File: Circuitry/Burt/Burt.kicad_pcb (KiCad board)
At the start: 2 copper layers, 111.1 x 114.2 mm, 41 parts, among them J1 Conn_01x20, J2 Conn_01x08_Female, M1 Motor_DC, Q1 SSM6N58NU, Q2 SSM6N58NU, Q3 SSM6N58NU, Q4 SSM6N58NU, Q5 SSM6N58NU, U1 MCP9701A, U2 A3908, U3 MCP73831-DFN, U4 74HC595

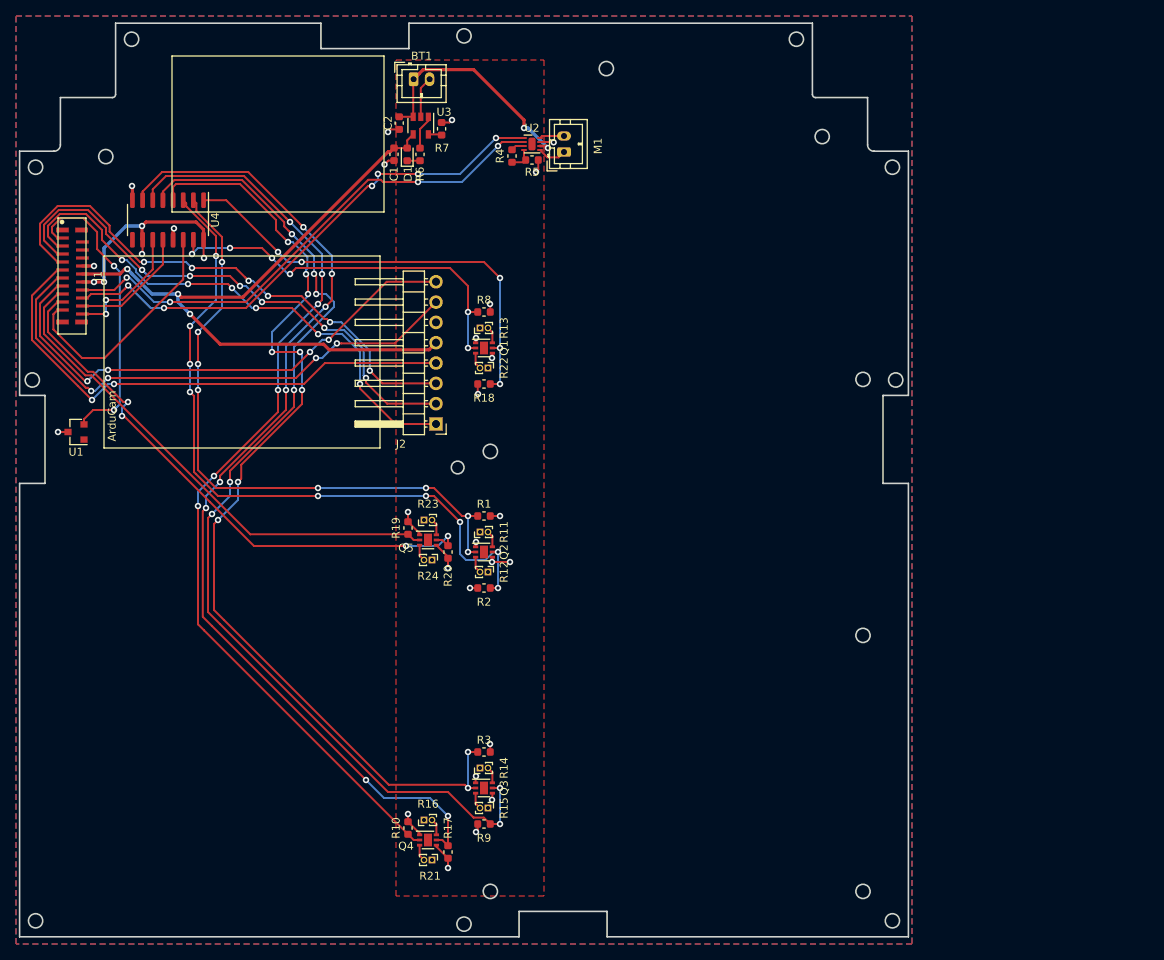
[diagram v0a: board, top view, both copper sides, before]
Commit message: Finshed lt surge layout
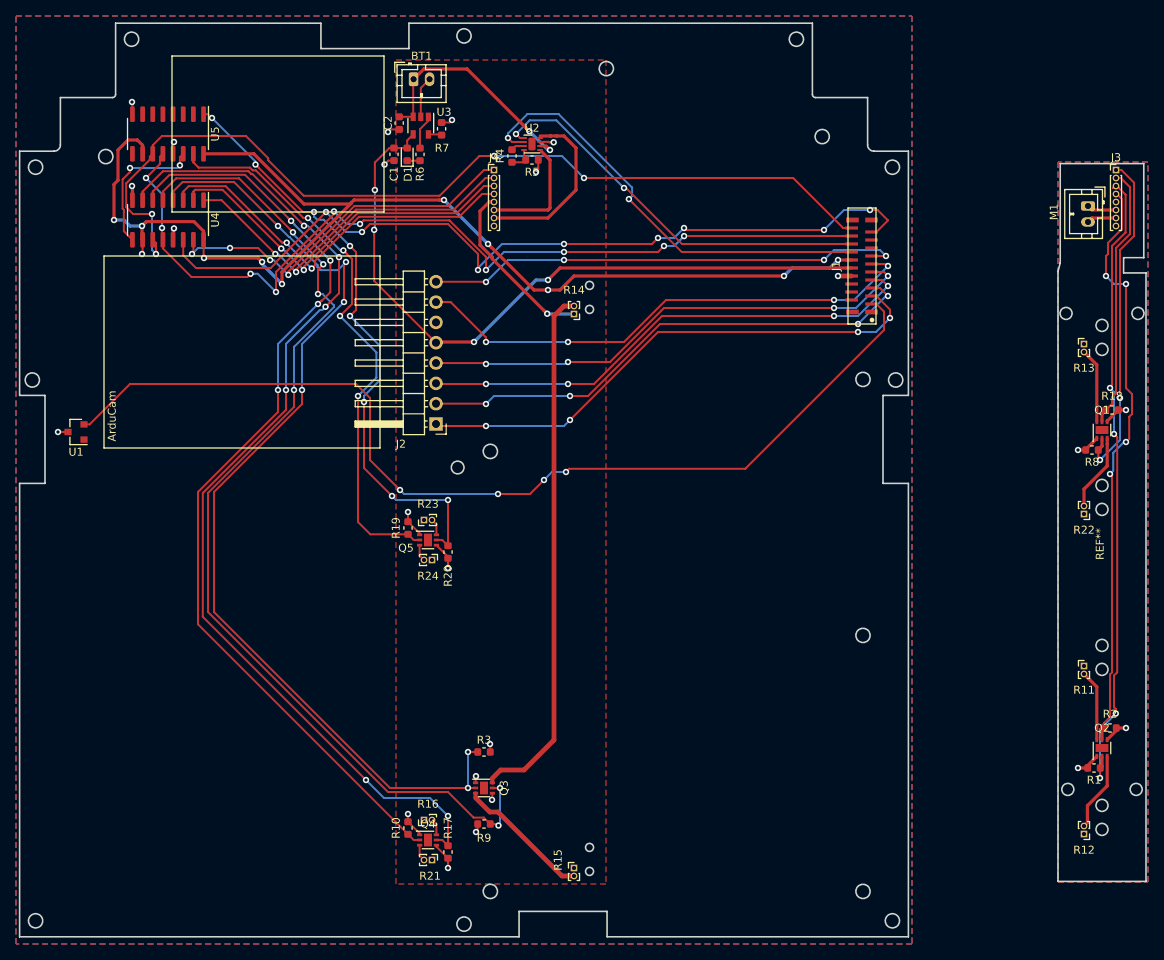
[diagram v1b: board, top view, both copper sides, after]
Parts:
- added J3: Conn_01x08_Male, Connector_PinHeader_1.00mm:PinHeader_1x08_P1.00mm_Vertical, F.Cu at (81.5, -46.8)
- added J4: Conn_01x08_Female, Connector_PinHeader_1.00mm:PinHeader_1x08_P1.00mm_Vertical, F.Cu at (3.75, -46.8)
- added REF**: Launcher, Custom:Launcher, F.Cu at (80.0, 0.00)
- added U5: 74HC595, Package_SO:SOIC-16_3.9x9.9mm_P1.27mm, F.Cu at (-37.0, -51.2)
- moved J1 98.8 mm to (49.8, -34.8), turned to 270 degrees
- moved R1 82.5 mm to (78.8, 28.0), turned to 0 degrees
- moved R12 81.4 mm to (77.5, 36.2), turned to 180 degrees
- moved Q2 81.0 mm to (79.8, 25.5), turned to 90 degrees
- moved R2 80.2 mm to (80.8, 23.0), turned to 180 degrees
- moved R18 78.6 mm to (81.0, -16.8), turned to 180 degrees
- moved R8 77.9 mm to (78.5, -11.8), turned to 0 degrees
- moved Q1 77.9 mm to (79.8, -14.2), turned to 90 degrees
- moved R11 77.3 mm to (77.5, 15.2), turned to 0 degrees
- moved R22 76.7 mm to (77.5, -3.75), turned to 180 degrees
- moved R13 75.5 mm to (77.5, -25.0), turned to 0 degrees
- moved M1 65.8 mm to (78.0, -42.2), turned to 270 degrees
- moved R14 58.0 mm to (13.8, -28.8), turned to 180 degrees
- moved R15 13.1 mm to (13.8, 40.5), turned to 0 degrees
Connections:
- net /BL7 renamed /BP3
- net /BL8 renamed /BP4
- J1 pad 18: Net-(J1-Pad18) -> (no net)
- J1 pad 19: Net-(J1-Pad19) -> (no net)
- J1 pad 20: Net-(J1-Pad20) -> (no net)
- J1 pad 8: /BP1 -> (no net)
- J1 pad 9: /BP2 -> (no net)
- M1 pad 1: Net-(M1-Pad1) -> /MOT_OUT_A
- M1 pad 2: Net-(M1-Pad2) -> /MOT_OUT_B
- Q1 pad 1: GND -> /GND_OUT
- Q1 pad 2: /BL1 -> /BL_OUT_1
- Q1 pad 4: GND -> /GND_OUT
- Q1 pad 5: /BL2 -> /BL_OUT_2
- Q2 pad 1: GND -> /GND_OUT
- Q2 pad 2: /BL3 -> /BL_OUT_3
- Q2 pad 4: GND -> /GND_OUT
- Q2 pad 5: /BL4 -> /BL_OUT_4
- R1 pad 1: GND -> /GND_OUT
- R1 pad 2: /BL3 -> /BL_OUT_3
- R11 pad 1: +BATT -> /BATT_OUT
- R12 pad 1: +BATT -> /BATT_OUT
- R13 pad 1: +BATT -> /BATT_OUT
- R18 pad 1: GND -> /GND_OUT
- R18 pad 2: /BL2 -> /BL_OUT_2
- R2 pad 1: GND -> /GND_OUT
- R2 pad 2: /BL4 -> /BL_OUT_4
- R22 pad 1: +BATT -> /BATT_OUT
- R8 pad 1: GND -> /GND_OUT
- R8 pad 2: /BL1 -> /BL_OUT_1
- U2 pad 1: Net-(M1-Pad2) -> /MOT_B
- U2 pad 4: Net-(M1-Pad1) -> /MOT_A
- U4 pad 9: Net-(U4-Pad9) -> /QH'
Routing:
- net +3V3: track 28.3 -> 148.1 mm, vias 5 -> 11
- net /SRCLK: track 15.8 -> 116.7 mm, vias 2 -> 4
- net /RCLK: track 15.3 -> 114.2 mm, vias 0 -> 10
- net /TEMP: track 37.7 -> 125.1 mm, vias 2 -> 4
- net /BL_OUT_3: track 0.00 -> 80.3 mm, vias 0 -> 4
- net /SER: track 30.0 -> 105.3 mm, vias 0 -> 8
- net /BL_OUT_4: track 0.00 -> 73.5 mm, vias 0 -> 4
- net Net-(Q3-Pad6): track 2.08 -> 66.3 mm
- net /BL_OUT_1: track 0.00 -> 42.3 mm, vias 0 -> 2
- net /BL4: track 88.7 -> 48.7 mm, vias 9 -> 2
- net /BL_OUT_2: track 0.00 -> 33.0 mm
- net /BL3: track 79.2 -> 47.5 mm, vias 8 -> 2
- net /MOT_B: track 0.00 -> 22.3 mm
- net +BATT: track 29.5 -> 51.6 mm, vias 2 -> 3
- net /QH': track 0.00 -> 17.9 mm, vias 0 -> 2
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- added copper zone on F.Cu, net /BATT_OUT
- added copper zone on B.Cu, net /GND_OUT
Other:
- outline, holes or cut-outs redrawn
- board text added: "TOP (Towards Open Face)"
